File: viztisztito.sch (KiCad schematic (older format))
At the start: 6 parts, among them P1 WATER_LEVEL_CONN, P2 BOARD_CONN, P3 SSR&PWR, P5 CONN_01X04, P6 CONN_01X02, P9 CONN_01X10

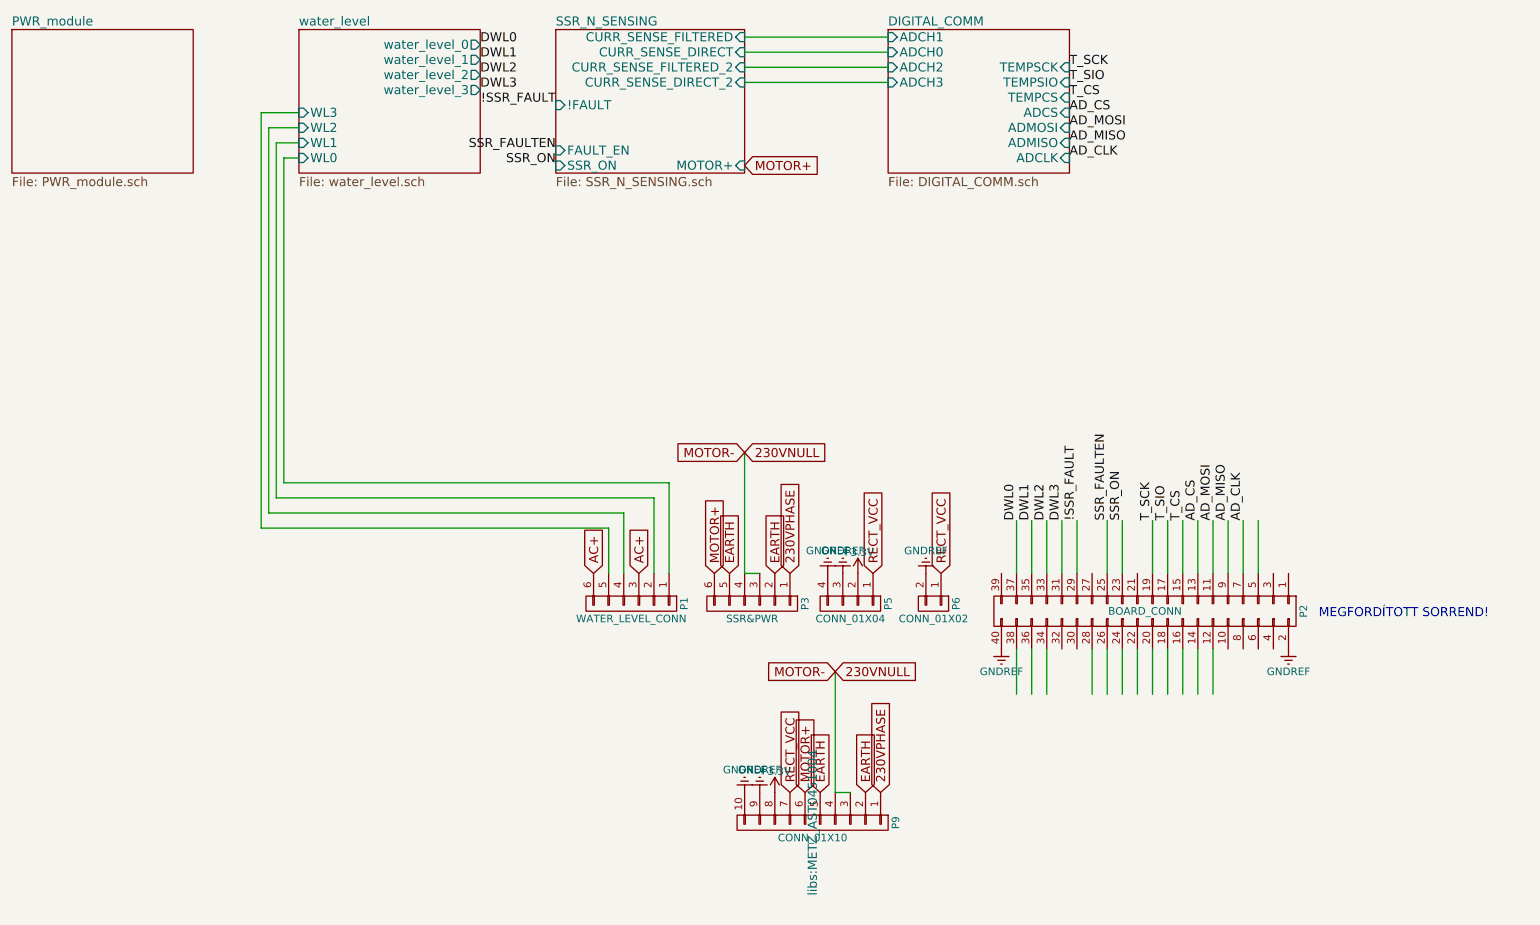
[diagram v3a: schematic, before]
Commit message: maybe final
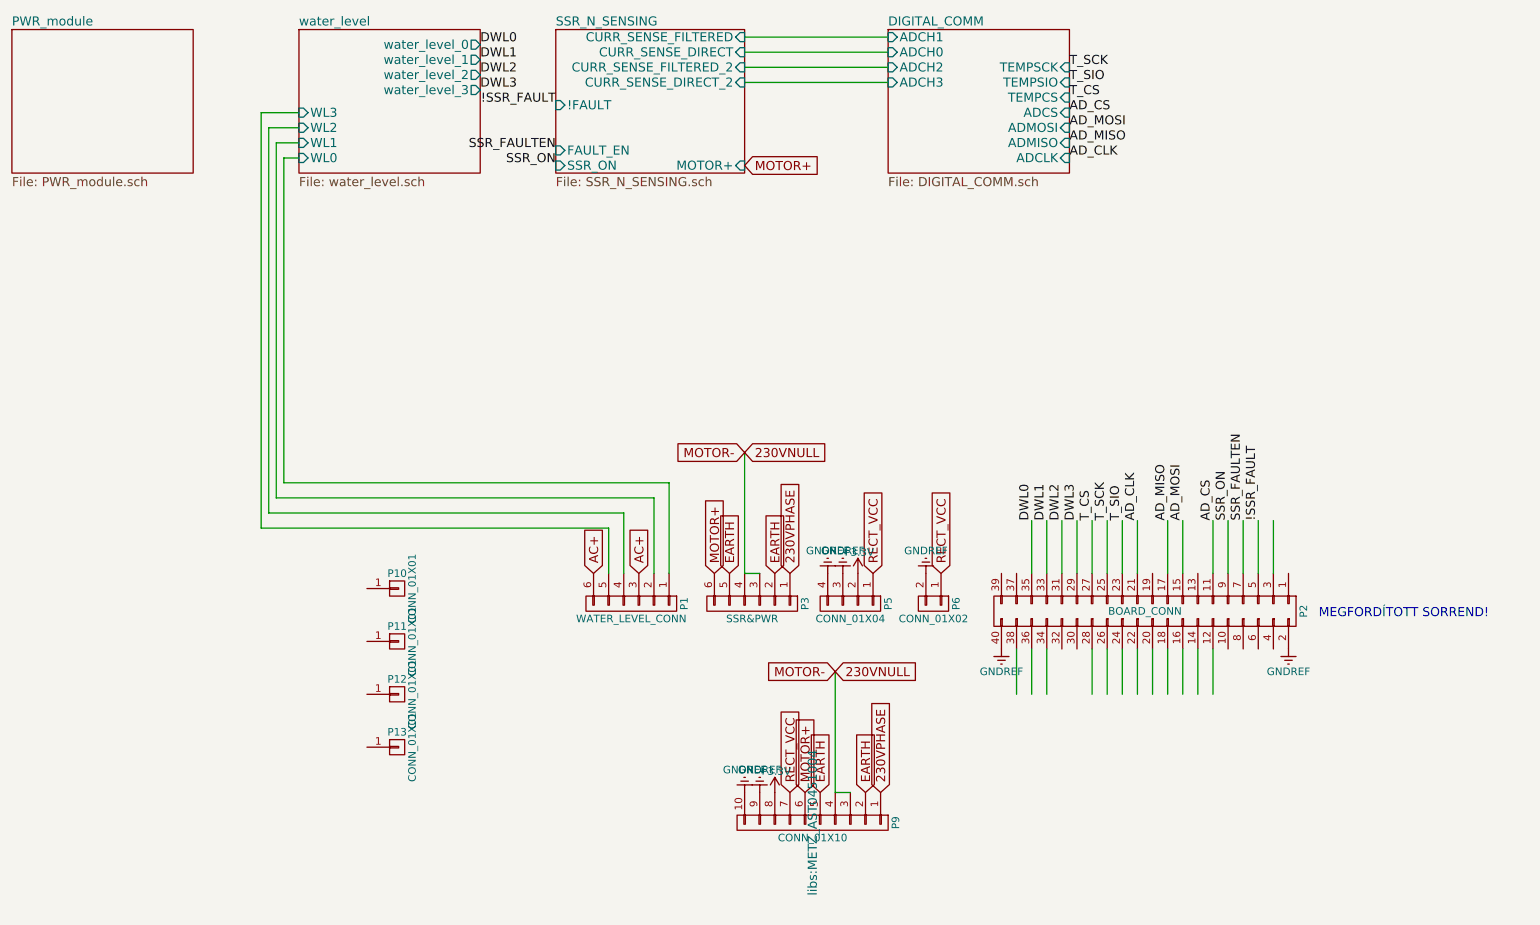
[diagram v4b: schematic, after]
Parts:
- added P10, P11, P12, P13: CONN_01X01, Mounting_Holes:MountingHole_4-5mm, symbol CONN_01X01
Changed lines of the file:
@@
 	7900 5100 7900 5400
 Wire Wire Line
-	7900 4600 7900 4250
-Wire Wire Line
 	8000 4600 8000 4250
 Wire Wire Line
@@
 	8600 4600 8600 4250
 Wire Wire Line
-	8800 4600 8800 4250
-Wire Wire Line
 	8900 4600 8900 4250
 Wire Wire Line
 	9000 4600 9000 4250
-Wire Wire Line
-	9100 4600 9100 4250
 Wire Wire Line
 	9200 4600 9200 4250
@@
 Text Label 8250 1850 0    60   ~ 0
 AD_CLK
-Text Label 7900 4250 1    60   ~ 0
+Text Label 8000 4250 1    60   ~ 0
 DWL0
-Text Label 8000 4250 1    60   ~ 0
+Text Label 8100 4250 1    60   ~ 0
 DWL1
-Text Label 8100 4250 1    60   ~ 0
+Text Label 8200 4250 1    60   ~ 0
 DWL2
-Text Label 8200 4250 1    60   ~ 0
+Text Label 8300 4250 1    60   ~ 0
 DWL3
-Text Label 8300 4250 1    60   ~ 0
+Text Label 9500 4250 1    60   ~ 0
 !SSR_FAULT
+Text Label 9400 4250 1    60   ~ 0
+SSR_FAULTEN
+Text Label 9300 4250 1    60   ~ 0
+SSR_ON
 Text Label 8500 4250 1    60   ~ 0
-SSR_FAULTEN
+T_SCK
 Text Label 8600 4250 1    60   ~ 0
-SSR_ON
-Text Label 8800 4250 1    60   ~ 0
-T_SCK
+T_SIO
+Text Label 8400 4250 1    60   ~ 0
+T_CS
+Text Label 9200 4250 1    60   ~ 0
+AD_CS
+Text Label 9000 4250 1    60   ~ 0
+AD_MOSI
 Text Label 8900 4250 1    60   ~ 0
-T_SIO
-Text Label 9000 4250 1    60   ~ 0
-T_CS
-Text Label 9100 4250 1    60   ~ 0
-AD_CS
-Text Label 9200 4250 1    60   ~ 0
-AD_MOSI
-Text Label 9300 4250 1    60   ~ 0
 AD_MISO
-Text Label 9400 4250 1    60   ~ 0
+Text Label 8700 4250 1    60   ~ 0
 AD_CLK
 Text Notes 9900 4900 0    60   ~ 0
@@
 	1    0    0    -1
 $EndComp
+Text GLabel 6900 6050 1    60   Input ~ 0
+EARTH
+Text GLabel 6500 6050 1    60   Input ~ 0
+MOTOR+
+Text GLabel 6700 5250 0    60   Input ~ 0
+MOTOR-
+Text GLabel 6600 6050 1    60   Input ~ 0
+EARTH
+Wire Wire Line
+	6700 5250 6700 6050
+Wire Wire Line
+	6700 6050 6800 6050
+Text GLabel 7000 6050 1    60   Input ~ 0
+230VPHASE
+Text GLabel 6700 5250 2    60   Input ~ 0
+230VNULL
+$Comp
+L CONN_01X01 P12
+U 1 1 562A651D
+P 3800 5400
+F 0 "P12" H 3800 5500 50  0000 C CNN
+F 1 "CONN_01X01" V 3900 5400 50  0000 C CNN
+F 2 "Mounting_Holes:MountingHole_4-5mm" H 3800 5400 60  0001 C CNN
+F 3 "" H 3800 5400 60  0000 C CNN
+	1    3800 5400
+	1    0    0    -1
+$EndComp
+$Comp
+L CONN_01X01 P11
+U 1 1 562A65E7
+P 3800 5050
+F 0 "P11" H 3800 5150 50  0000 C CNN
+F 1 "CONN_01X01" V 3900 5050 50  0000 C CNN
+F 2 "Mounting_Holes:MountingHole_4-5mm" H 3800 5050 60  0001 C CNN
+F 3 "" H 3800 5050 60  0000 C CNN
+	1    3800 5050
+	1    0    0    -1
+$EndComp
+$Comp
+L CONN_01X01 P10
+U 1 1 562A66C7
+P 3800 4700
+F 0 "P10" H 3800 4800 50  0000 C CNN
+F 1 "CONN_01X01" V 3900 4700 50  0000 C CNN
+F 2 "Mounting_Holes:MountingHole_4-5mm" H 3800 4700 60  0001 C CNN
+F 3 "" H 3800 4700 60  0000 C CNN
+	1    3800 4700
+	1    0    0    -1
+$EndComp
+$Comp
+L CONN_01X01 P13
+U 1 1 562A67A4
+P 3800 5750
+F 0 "P13" H 3800 5850 50  0000 C CNN
+F 1 "CONN_01X01" V 3900 5750 50  0000 C CNN
+F 2 "Mounting_Holes:MountingHole_4-5mm" H 3800 5750 60  0001 C CNN
+F 3 "" H 3800 5750 60  0000 C CNN
+	1    3800 5750
+	1    0    0    -1
+$EndComp
+Wire Wire Line
+	9600 4600 9600 4250
+Wire Wire Line
+	8700 4600 8700 4250
+Wire Wire Line
+	8400 4600 8400 4250
 $Comp
 L GNDREF #PWR09
@@
 	-1   0    0    1
 $EndComp
-Text GLabel 6900 6050 1    60   Input ~ 0
-EARTH
-Text GLabel 6500 6050 1    60   Input ~ 0
-MOTOR+
-Text GLabel 6700 5250 0    60   Input ~ 0
-MOTOR-
-Text GLabel 6600 6050 1    60   Input ~ 0
-EARTH
-Wire Wire Line
-	6700 5250 6700 6050
-Wire Wire Line
-	6700 6050 6800 6050
-Text GLabel 7000 6050 1    60   Input ~ 0
-230VPHASE
-Text GLabel 6700 5250 2    60   Input ~ 0
-230VNULL
 $EndSCHEMATC
